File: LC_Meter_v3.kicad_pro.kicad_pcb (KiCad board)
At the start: 2 copper layers, 50.2 x 50 mm, 38 parts, among them J1 TEST, J2 Conn_DC-IN, J3 DC_SEL, J4 Conn_i2c LCD, J5 Conn_i2c LCD2, P1 COM, SW1 SW_DPDT_x2, SW2 SW_DIP_x02, SW3 RESET, U1 74HCU04, U2 LM78M05_TO220, U3 ATmega328P-PU, Y1 16MHz

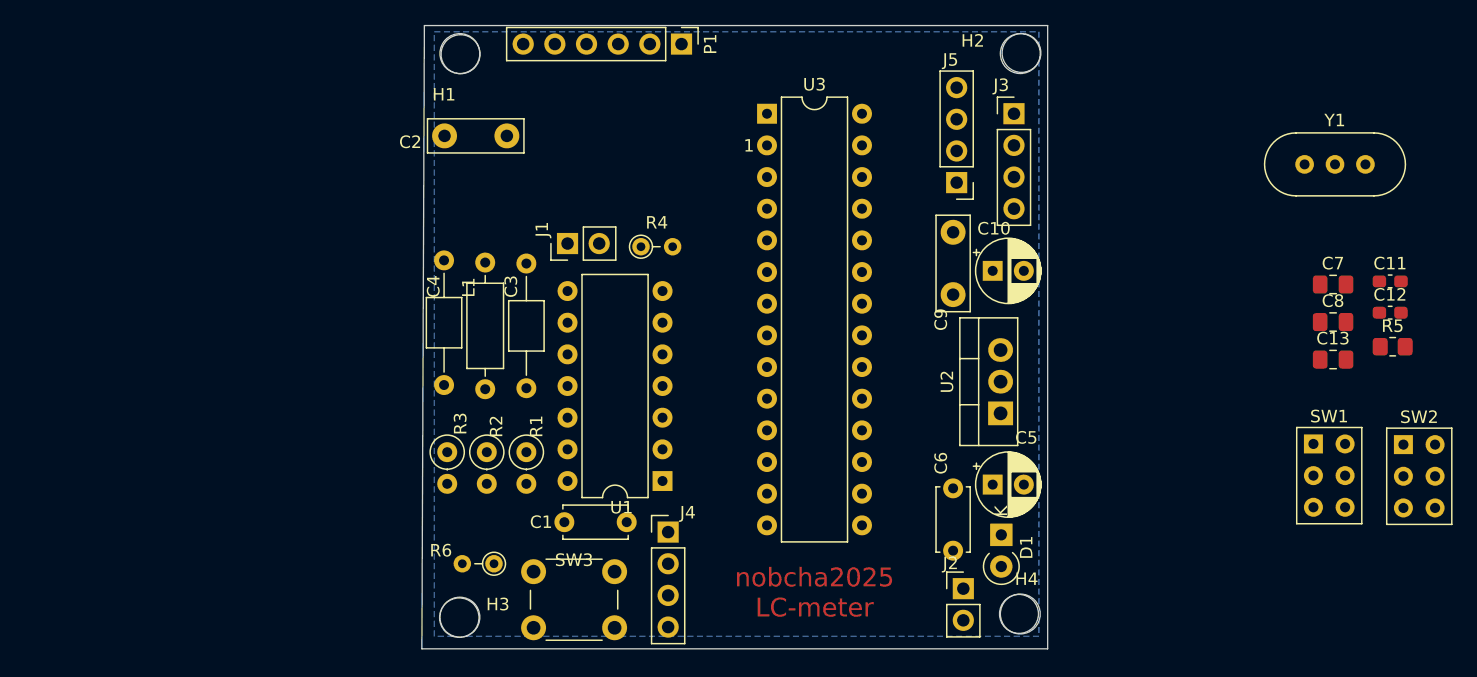
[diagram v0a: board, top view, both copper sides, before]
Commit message: Advanced design V1
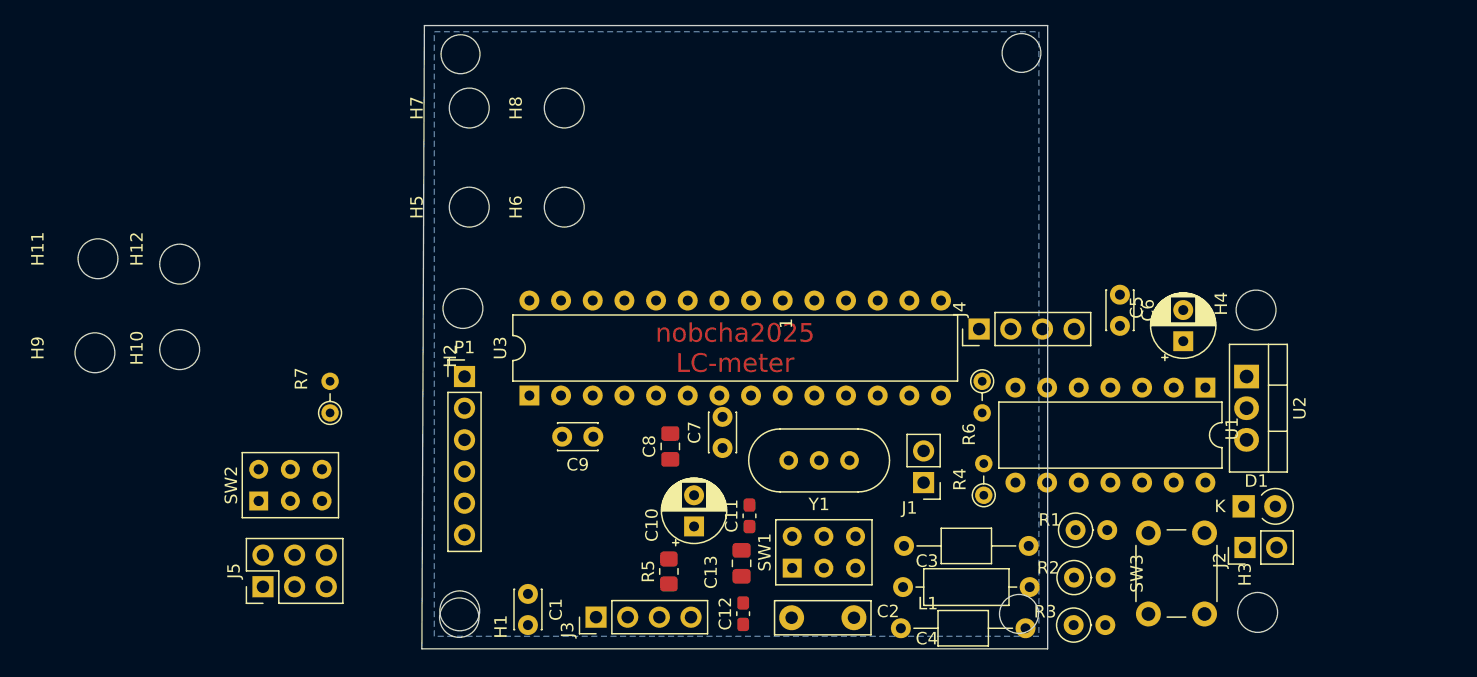
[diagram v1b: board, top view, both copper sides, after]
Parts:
- added H10: MountingHole3.2, MountingHole:MountingHole_3.2mm_M3, F.Cu at (96.1, 87.6)
- added H11: MountingHole3.2, MountingHole:MountingHole_3.2mm_M3, F.Cu at (89.5, 80.3)
- added H12: MountingHole3.2, MountingHole:MountingHole_3.2mm_M3, F.Cu at (96.1, 80.7)
- added H5: MountingHole3.2, MountingHole:MountingHole_3.2mm_M3, F.Cu at (119.3, 76.2)
- added H6: MountingHole3.2, MountingHole:MountingHole_3.2mm_M3, F.Cu at (126.9, 76.2)
- added H7: MountingHole3.2, MountingHole:MountingHole_3.2mm_M3, F.Cu at (119.3, 68.2)
- added H8: MountingHole3.2, MountingHole:MountingHole_3.2mm_M3, F.Cu at (126.9, 68.2)
- added H9: MountingHole3.2, MountingHole:MountingHole_3.2mm_M3, F.Cu at (89.3, 87.9)
- added R7: 10k, Resistor_THT:R_Axial_DIN0204_L3.6mm_D1.6mm_P2.54mm_Vertical, F.Cu at (108.1, 92.7)
- C1, C6: footprint Capacitor_THT:C_Disc_D5.0mm_W2.5mm_P5.00mm -> Capacitor_THT:C_Disc_D3.0mm_W2.0mm_P2.50mm
- C7: footprint Capacitor_SMD:C_0805_2012Metric_Pad1.18x1.45mm_HandSolder -> Capacitor_THT:C_Disc_D3.0mm_W2.0mm_P2.50mm
- C9: footprint Capacitor_THT:C_Disc_D7.5mm_W2.5mm_P5.00mm -> Capacitor_THT:C_Disc_D3.0mm_W2.0mm_P2.50mm
- J5: value Conn_i2c LCD2 -> ICSP; footprint Connector_PinHeader_2.54mm:PinHeader_1x04_P2.54mm_Vertical -> Connector_PinHeader_2.54mm:PinHeader_2x03_P2.54mm_Vertical
- SW2: value SW_DIP_x02 -> SW_DPDT_x2
- moved SW2 91.9 mm to (102.4, 99.7), turned to 90 degrees
- moved J5 64.4 mm to (102.8, 106.6), turned to 90 degrees
- moved H3 64.0 mm to (182.5, 108.7), turned to 90 degrees
- moved R5 60.8 mm to (135.3, 105.4), turned to 90 degrees
- moved C12 57.2 mm to (141.3, 108.8), turned to 90 degrees
- moved C11 54.7 mm to (141.8, 100.9), turned to 90 degrees
- moved C8 54.1 mm to (135.4, 95.4), turned to 90 degrees
- moved J3 52.5 mm to (129.5, 109.1), turned to 90 degrees
- moved R3 52.1 mm to (167.8, 109.7), turned to 0 degrees
- moved C2 50.7 mm to (150.2, 109.1), turned to 180 degrees
- moved C7 50.7 mm to (139.6, 95.5), turned to 90 degrees
- moved C4 50.6 mm to (163.9, 109.9), turned to 180 degrees
- moved C13 50.2 mm to (141.1, 104.7), turned to 90 degrees
- moved SW3 49.4 mm to (173.8, 108.8), turned to 90 degrees
- moved H2 49.2 mm to (118.8, 84.3), turned to 90 degrees
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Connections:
- C3 pad 1: Net-(C3-Pad1) -> Net-(SW2B-A)
- J5 pad 1: +5V -> /12(MISO)
- J5 pad 2: /A5 -> /13(SCK)
- J5 pad 3: /A4 -> /Reset
- SW2 pad 2: Net-(C3-Pad1) -> GND
- SW2 pad 3: GND -> unconnected-(SW2A-C-Pad3)
- SW2 pad 4: GND -> Net-(SW2B-A)
- SW2 pad 5: (no net) -> GND
- SW2 pad 6: (no net) -> unconnected-(SW2B-C-Pad6)
